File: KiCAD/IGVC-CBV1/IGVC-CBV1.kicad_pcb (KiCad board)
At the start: 2 copper layers, 4.5 x 9.8 mm, 46 parts, among them IC1 STM32F407ZGT6, IC2 SPX3819M5-L-3-3_TR, IC3 AT45DB081E-SSHN-B, J1 STLINKV2 PINS (2.54mm Pitch), J2 Motor Driver Pins (2.54mm Pit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, J3 12401948E412A, J4 Conn_01x02, J5 Screw_Terminal_01x02, SW1 SW_SPDT, Y1 EB2532YA12-25.000M_TR

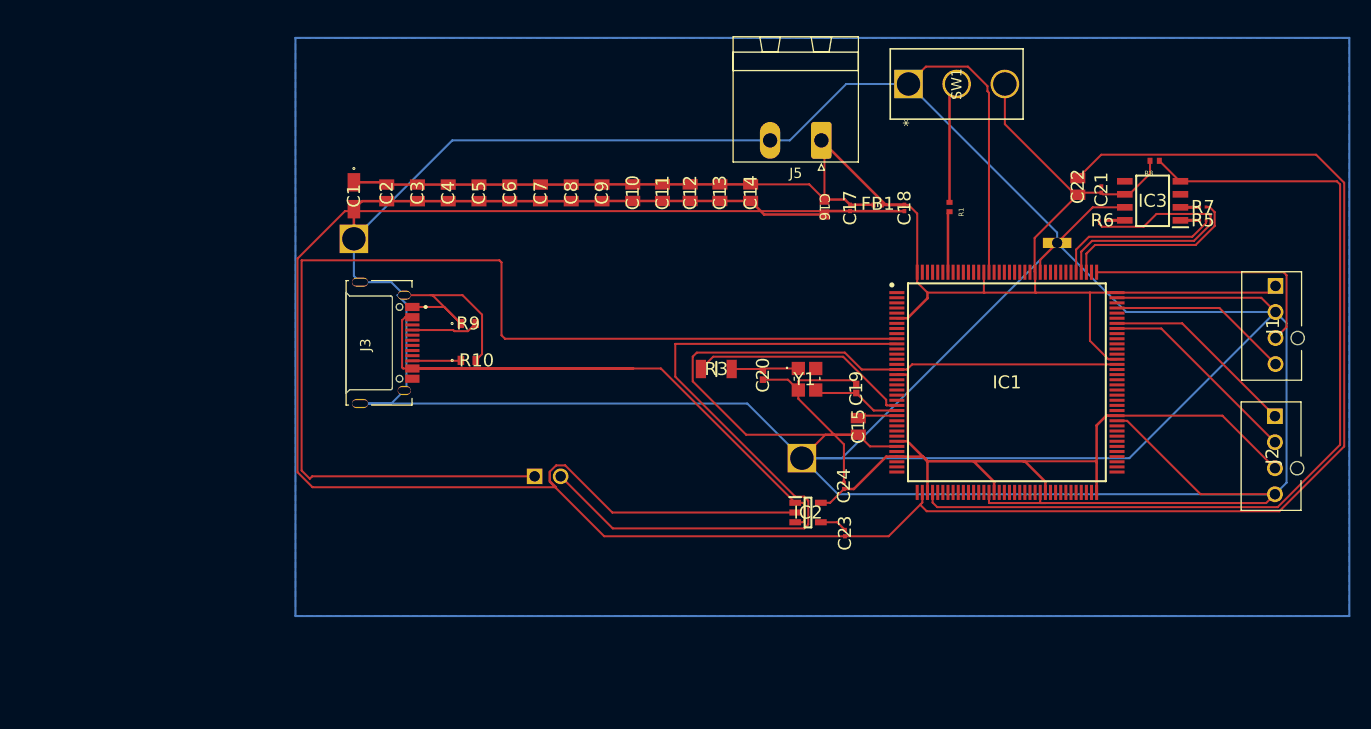
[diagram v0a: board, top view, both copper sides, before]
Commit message: PCB Update
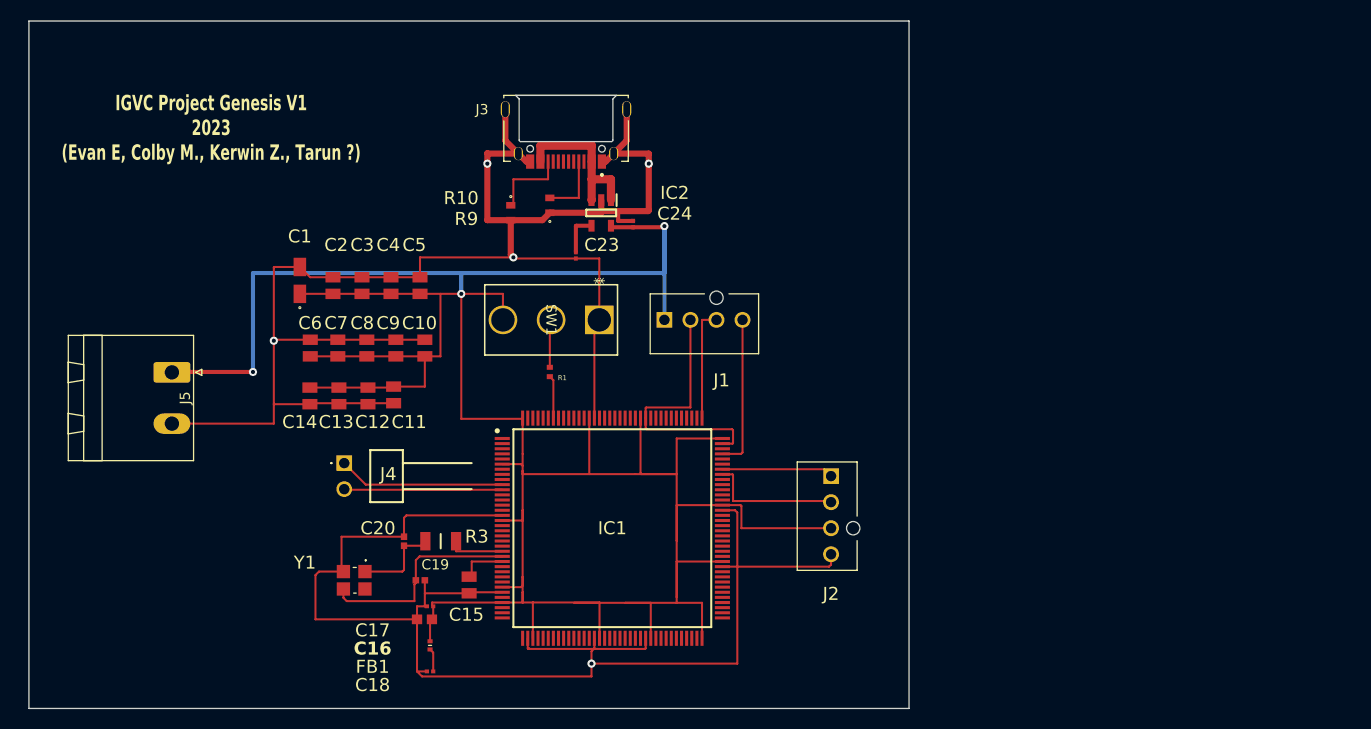
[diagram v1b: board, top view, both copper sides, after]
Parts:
- removed ? (x3): , 
- removed C21: 1uF, LIB_GRMMDXR60J105ME05D:CAPC0502X28N
- removed C22: .1uF, LIB_08051C104K4Z2A:CAPC2012X140N
- removed IC3: AT45DB081E-SSHN-B, LIB_AT45DB081E-SSHN-B:SOIC127P600X175-8N
- removed R5, R6, R7: 0 Ohm, LIB_ERJ-1GJ0R00C:ERJ1G_1023
- removed R8: 10k, RC0402FR-0710KL:RESC1005X40N
- J4: moved to F.Cu
- moved J5 67.3 mm to (115.6, 88.6), turned to -90 degrees
- moved C18 64.7 mm to (140.7, 117.8), turned to 180 degrees
- moved FB1 61.3 mm to (140.7, 115.3), turned to 90 degrees
- moved J1 59.7 mm to (163.6, 83.5), turned to 180 degrees
- moved C17 56.5 mm to (140.7, 111.4), turned to 180 degrees
- moved C16 56.0 mm to (140.2, 112.7), turned to 180 degrees
- moved Y1 48.3 mm to (133.3, 108.9), turned to -90 degrees
- moved C14 47.3 mm to (129.0, 90.9)
- moved C19 46.5 mm to (139.8, 108.9), turned to 180 degrees
- moved J2 43.7 mm to (179.8, 98.7)
- moved R1 42.2 mm to (152.4, 88.6)
- moved C13 42.1 mm to (131.8, 90.9)
- moved IC1 41.0 mm to (158.5, 103.8)
- moved C15 41.0 mm to (144.5, 109.4)
- moved C20 38.6 mm to (138.2, 105.1), turned to -90 degrees
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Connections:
- IC1 pad 111: SPI3_SCK -> unconnected-(IC1-PC10-Pad111)
- IC1 pad 112: SPI3_MISO -> unconnected-(IC1-PC11-Pad112)
- IC1 pad 113: SPI3_MOSI -> unconnected-(IC1-PC12-Pad113)
- IC1 pad 40: SPI3_NSS -> unconnected-(IC1-PA4-Pad40)
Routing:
- net GND: track 883.5 -> 316.4 mm, vias 0 -> 5
- net I2C2_SDA: track 109.1 -> 16.3 mm
- net SPI3_NSS: track 87.4 -> 0.00 mm
- net +3.3V: track 243.0 -> 309.5 mm, vias 0 -> 3
- net VBUS: track 74.6 -> 15.8 mm
- net I2C2_SCL: track 71.5 -> 15.4 mm
- net SPI3_MISO: track 28.5 -> 0.00 mm
- net SPI3_SCK: track 17.8 -> 0.00 mm
- net RCC_OSC_IN: track 21.9 -> 5.48 mm
- net SPI3_MOSI: track 16.2 -> 0.00 mm
- net SWCLK: track 25.2 -> 11.0 mm
- net RCC_OSC_OUT: track 8.74 -> 20.5 mm
- net USART1_RX: track 19.2 -> 10.9 mm
- net /SW_BOOT0: track 11.8 -> 4.68 mm
- net USART1_TX: track 20.0 -> 13.2 mm
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- removed copper zone on B.Cu, net GND
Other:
- board size 4.5 x 9.8 mm -> 85.9 x 67.1 mm
- board text added: "IGVC Project Genesis V1 2023 (Evan E, Colby M., Kerwin Z., Tarun ?)"
